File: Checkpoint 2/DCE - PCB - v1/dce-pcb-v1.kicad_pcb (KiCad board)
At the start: 2 copper layers, 190.4 x 110.6 mm, 51 parts, among them J1 Conn_01x06_Socket, J2 Conn_01x02_Socket, M1 2N7000, Q1 BC547B, Q2 BC547B, Q3 BC547B, Q4 BC557B, Q5 BC557B, Q6 BC547B, Q7 TIP41C, Q8 TIP42C, Q9 BC547B, U1 LM324

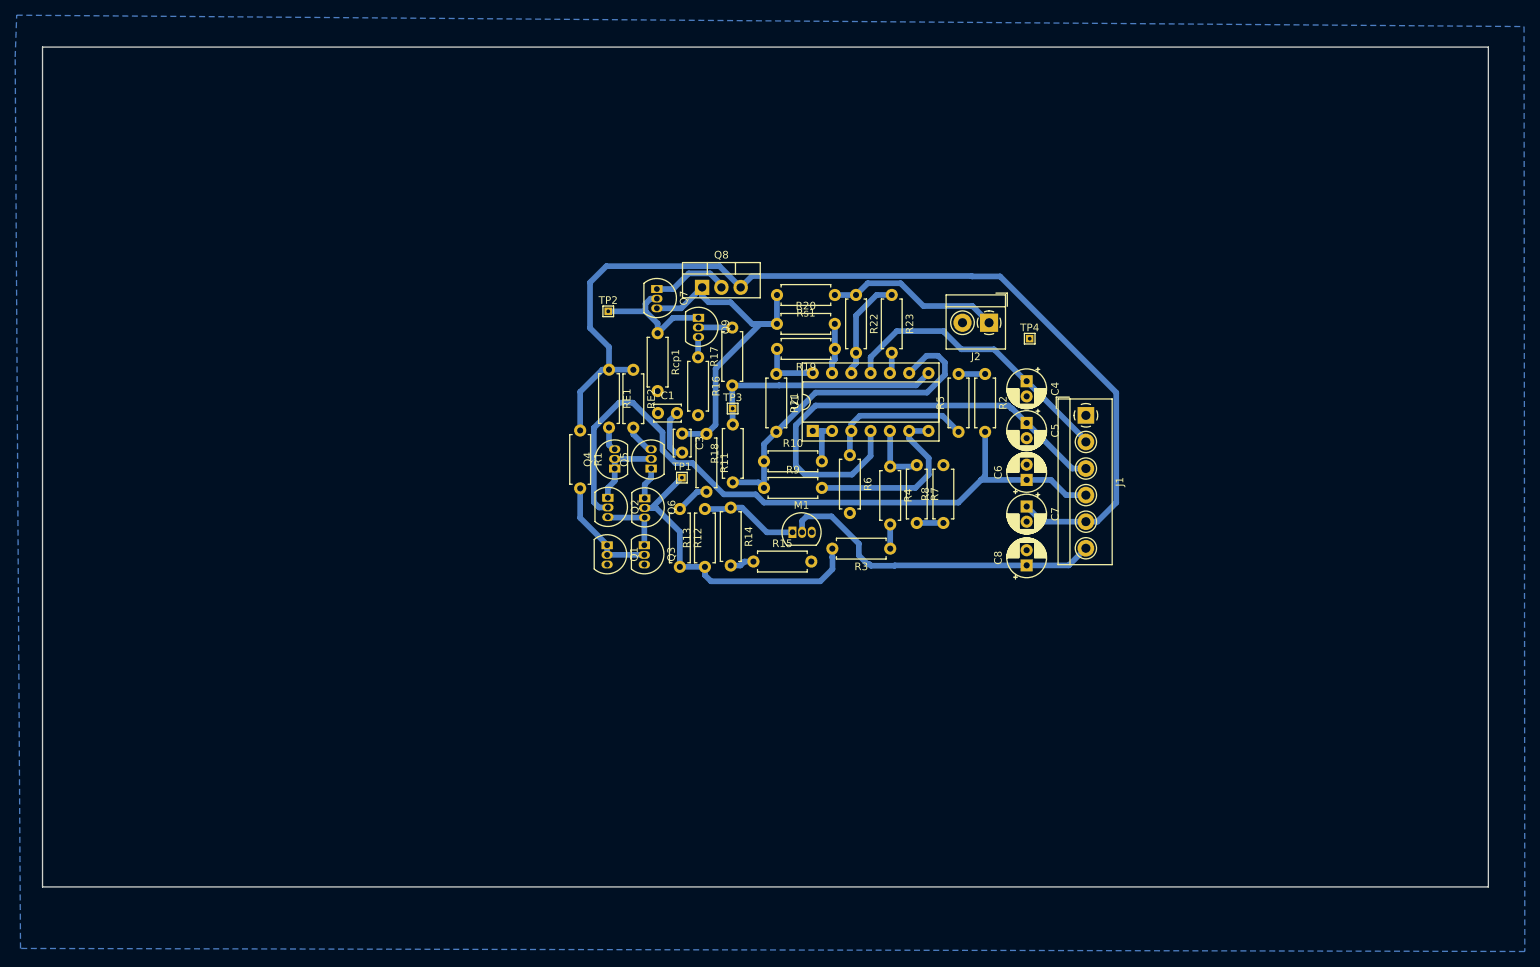
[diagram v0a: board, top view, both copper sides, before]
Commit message: Actualizacion PCB
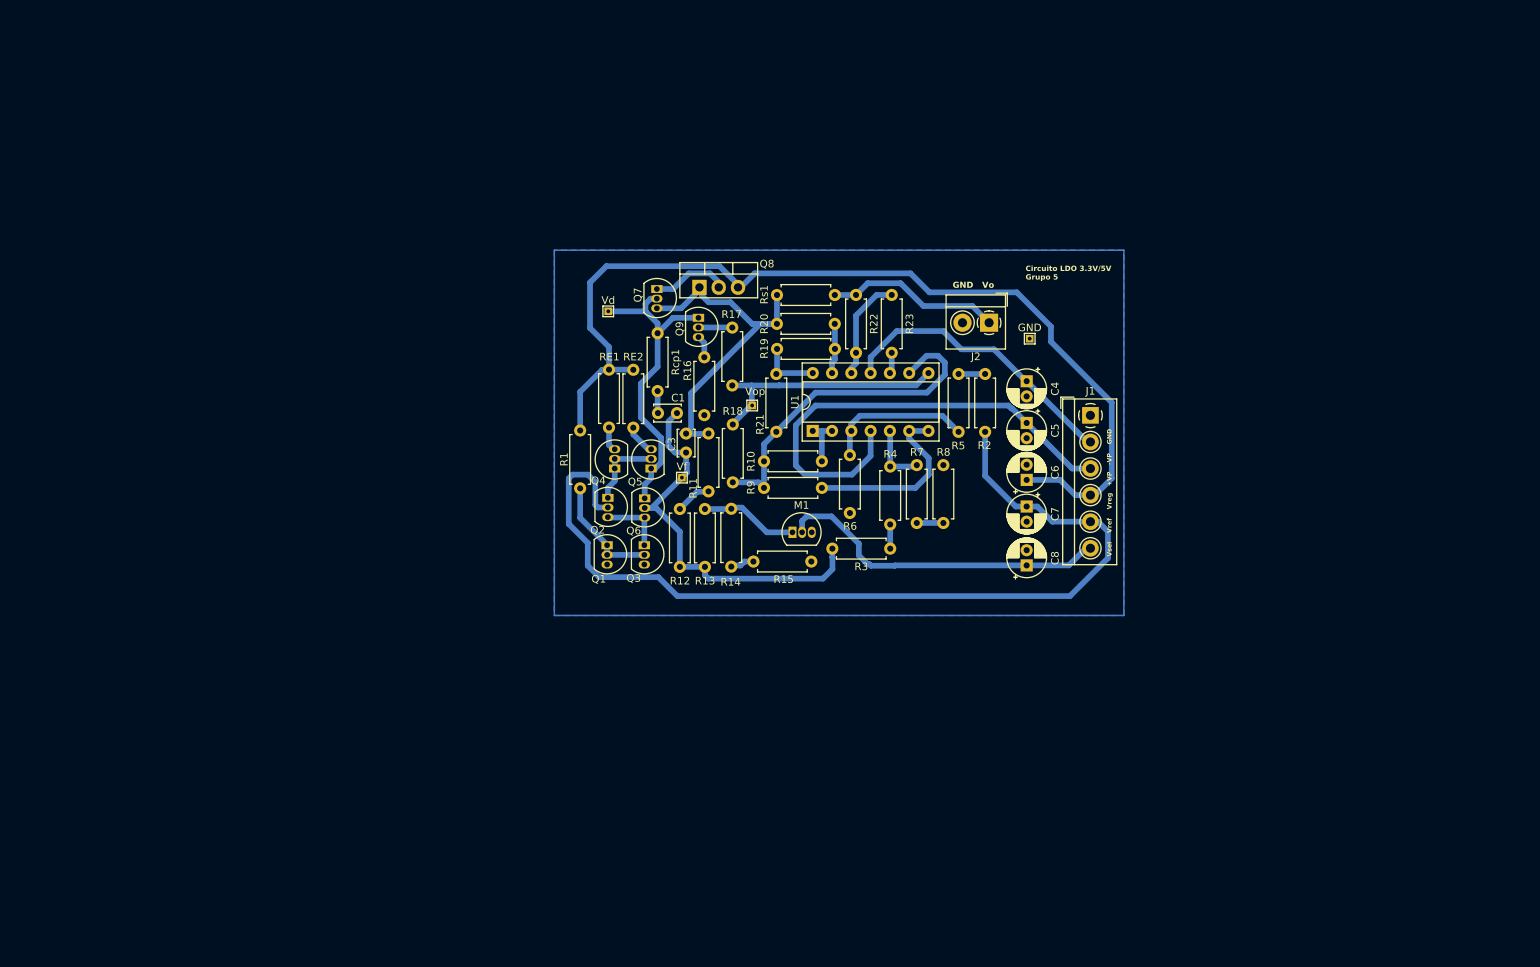
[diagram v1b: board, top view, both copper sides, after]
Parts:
- moved Vop 2.60 mm to (149.7, 67.9)
- moved R16 0.82 mm to (143.3, 61.5)
- moved J1 0.60 mm to (194.2, 69.2)
- moved C3 0.52 mm to (140.9, 71.6)
- moved Q8 0.35 mm to (142.7, 52.3)
- moved R11 0.27 mm to (143.9, 71.6)
- moved R14 0.17 mm to (146.9, 81.5)
- renumbered TP4 to GND, TP2 to Vd, TP1 to Vf, TP3 to Vop
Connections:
- C6 pad 1: /Vref -> /Vreg
- C7 pad 1: /Vreg -> /Vref
- J1 pad 4: /Vref -> /Vreg
- J1 pad 5: /Vreg -> /Vref
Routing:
- net /Vref: track 93.5 -> 122.2 mm
- net /Vlc: track 21.7 -> 42.4 mm
- net /Vreg: track 132.3 -> 128.5 mm
- net /Vf: track 48.8 -> 52.6 mm
- net Net-(C1-Pad1): track 0.00 -> 2.92 mm
- net Net-(Q7-E): track 46.2 -> 47.3 mm
- net Net-(R17-Pad1): track 31.7 -> 32.7 mm
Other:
- board outline removed
- board text added: "Circuito LDO 3.3V/5V Grupo 5"
- board text added: "GND Vo"
- board text added: "Vsel Vref Vreg +VP -VP GND"
